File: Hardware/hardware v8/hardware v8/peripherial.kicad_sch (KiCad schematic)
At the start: 9 parts, among them IC2 W25Q128JVPIQ_TR, IC4 MAX-M10S-00B

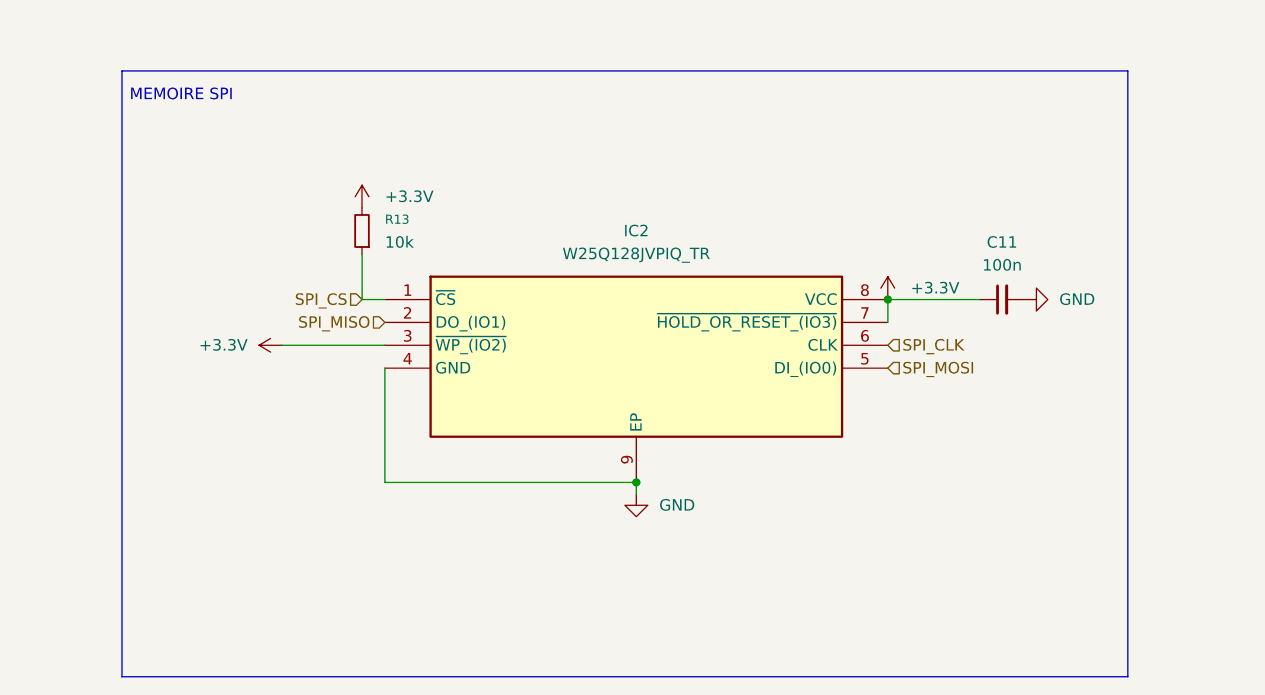
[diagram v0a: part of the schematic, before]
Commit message: v8
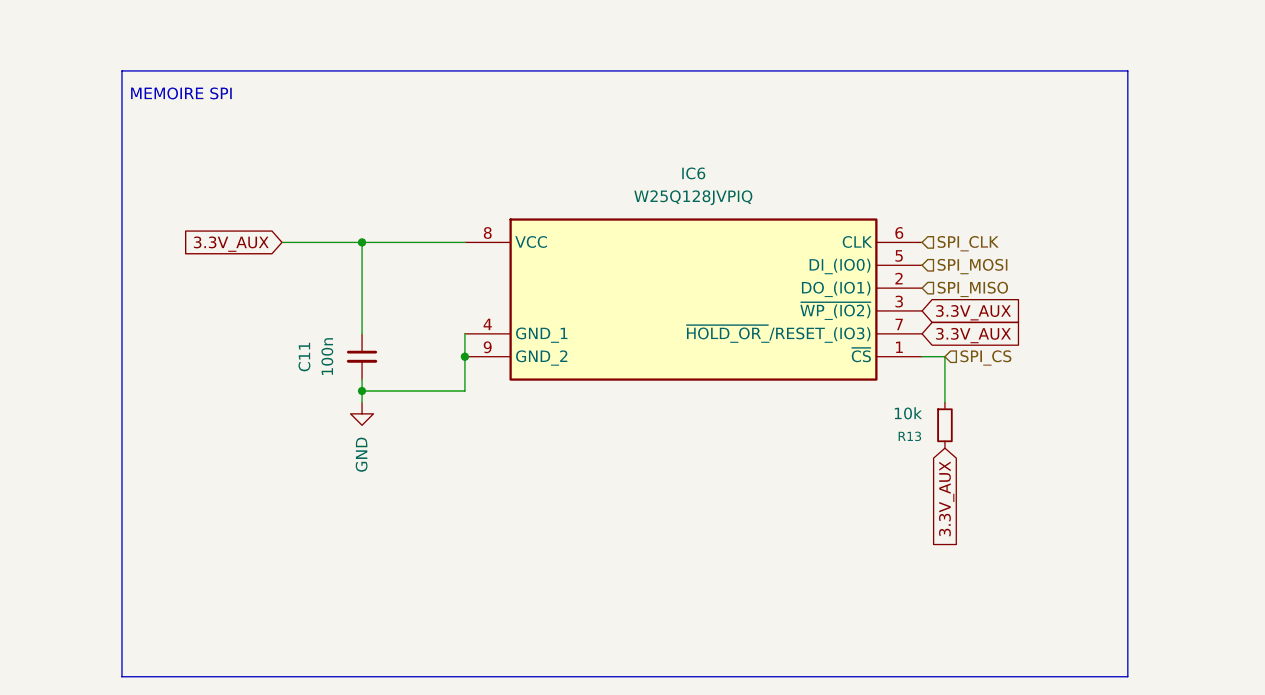
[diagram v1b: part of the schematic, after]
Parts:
- removed IC2: W25Q128JVPIQ_TR, w25q128:SON127P600X500X80-9N-D, symbol winbond:W25Q128JVPIQ_TR
- added IC6: W25Q128JVPIQ, samacsys2:SON127P600X500X80-9N-D, symbol samacsys2:W25Q128JVPIQ
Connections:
- net GND: now also IC6.4 (GND_1), IC6.9 (GND_2)
- net SPI_CLK: now also IC6.6 (CLK)
- net SPI_CS: now also IC6.1 (~{CS})
- net SPI_MISO: now also IC6.2 (DO_(IO1))
- net SPI_MOSI: now also IC6.5 (DI_(IO0))
- net +3.3V renamed 3.3V_AUX
- net 3.3V_AUX: now also IC6.3 (~{WP_(IO2)}), IC6.7 (~{HOLD_OR_}/RESET_(IO3)), IC6.8 (VCC)
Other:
- moved on the sheet: C11, R13
